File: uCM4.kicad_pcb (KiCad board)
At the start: 2 copper layers, 55 x 48 mm, 81 parts, among them IC1 MAX17048G+, J10 USB_C_Receptacle, J2 Micro_SD_Card_Det, J4 Conn_01x04, J5 DummyJ, J6 DummyJ, Q2 SI2369DS, SW1 SW_DIP_x01, SW3 SW_Push, SW4 SW_SPDT, U1 BNO055, U18 RT9742GGJ5, U2 SN74LVC1G07DBVR, U3 TPS3839DBZ, U4 TPS61022, U5 TPD2EUSB30, U6 TP4057, U7 HC-PM254-5.0H-2X7PS, U8 ADAU7002ACBZ-R7, U9 HC-PM254-5.0H-2X7PS

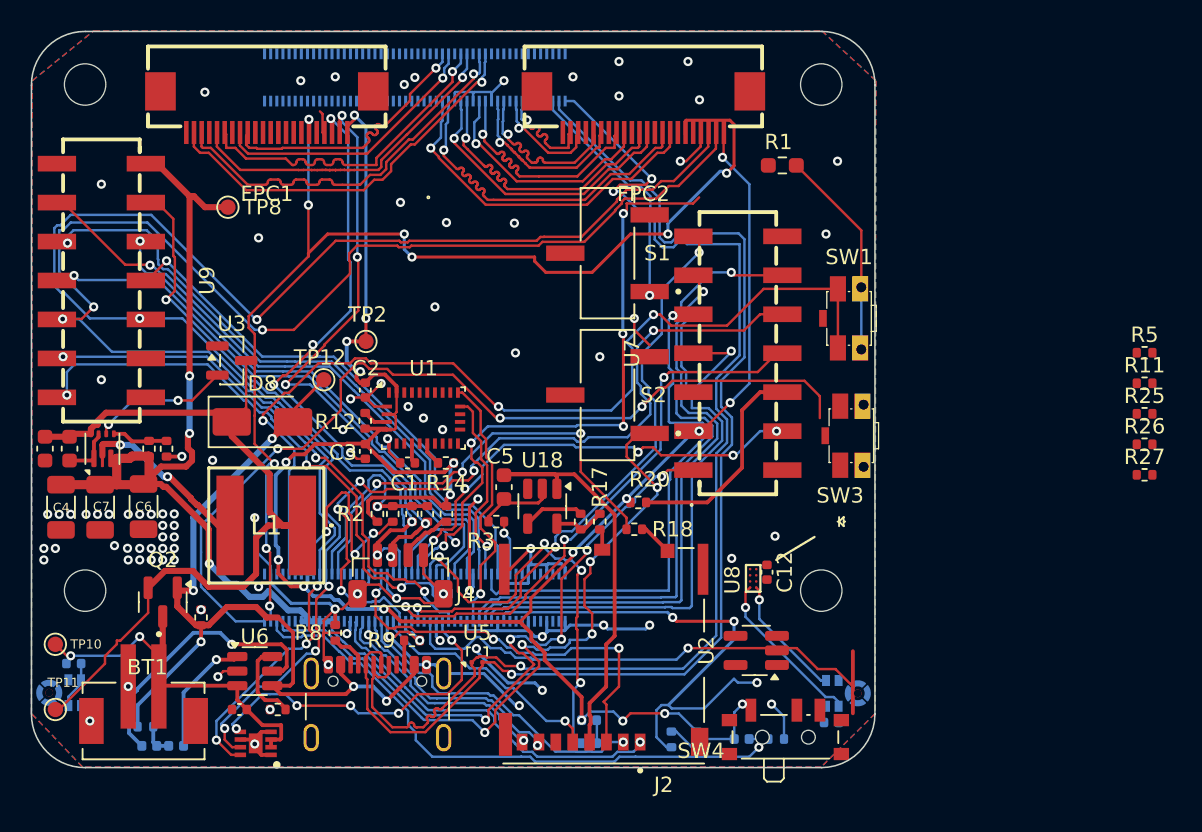
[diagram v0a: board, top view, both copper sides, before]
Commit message: Routing in progress
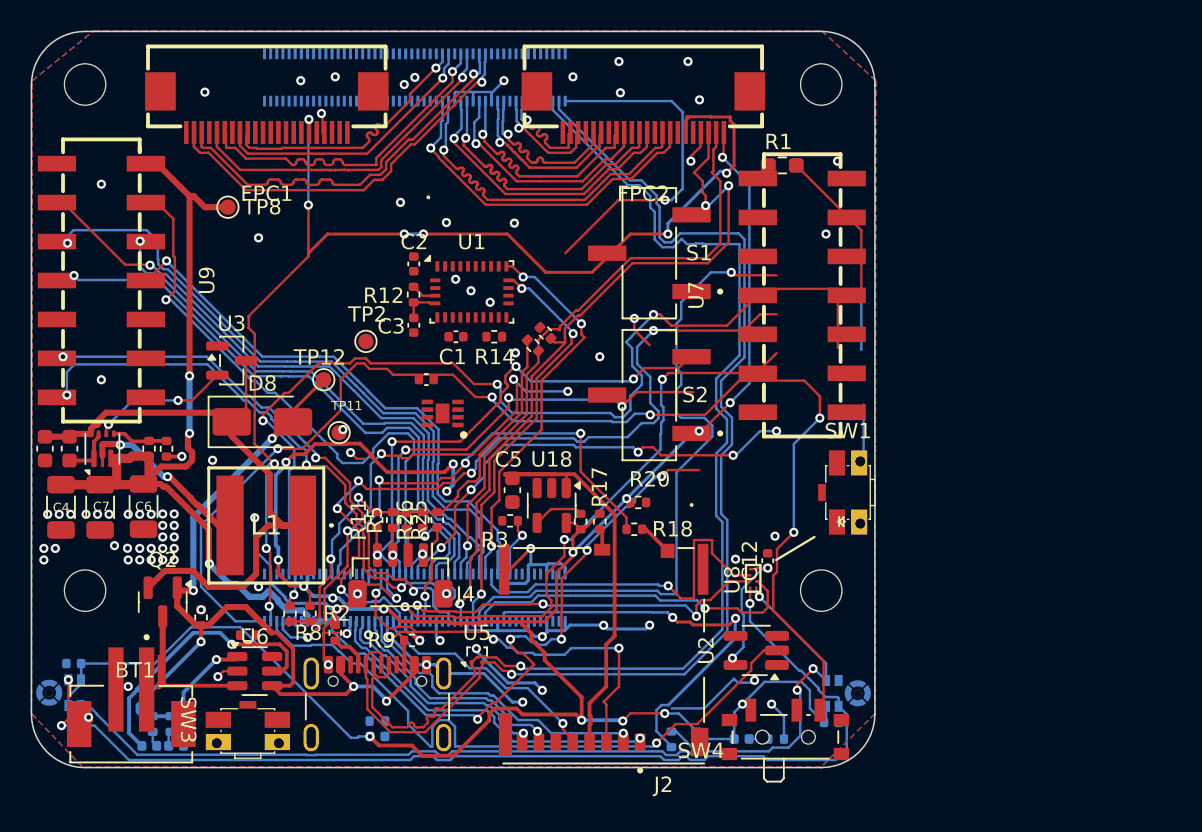
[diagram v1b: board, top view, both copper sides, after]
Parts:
- removed TP10: TestPoint, TestPoint:TestPoint_Pad_D1.0mm
- R27: moved to B.Cu
- moved R27 66.7 mm to (128.8, 130.2), turned to -90 degrees
- moved R11 50.9 mm to (143.4, 116.9), turned to 90 degrees
- moved R5 50.2 mm to (144.5, 116.9), turned to 90 degrees
- moved R26 47.3 mm to (146.4, 116.9), turned to 90 degrees
- moved R25 46.6 mm to (147.4, 116.9), turned to 90 degrees
- moved SW3 43.8 mm to (135.1, 130.7), turned to 0 degrees
- moved TP11 25.8 mm to (141.0, 111.2)
- moved C13 24.7 mm to (146.7, 107.7)
- moved IC1 24.7 mm to (147.8, 110.0)
- moved R7 14.7 mm to (154.4, 104.7), turned to 135 degrees
- moved R10 13.9 mm to (143.5, 130.0)
- moved D3 13.8 mm to (143.5, 131.0)
- moved R6 13.0 mm to (153.6, 105.5), turned to 135 degrees
- moved SW1 11.4 mm to (174.2, 115.1)
- moved R4 9.33 mm to (137.8, 123.0), turned to -90 degrees
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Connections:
- FPC2 pad 3: GND -> /SCL1
- Module1 pad 35: GND -> /SCL1
- R23 pad 1: +3V3 -> /GPIO_VREF
- R25 pad 2: Net-(R25-Pad2) -> /GPIO_VREF
- R26 pad 2: Net-(R25-Pad2) -> /GPIO_VREF
- R7 pad 1: GND -> /SCL1
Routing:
- net /SDA0: track 107.0 -> 0.00 mm, vias 6 -> 0
- net /SCL0: track 102.7 -> 0.00 mm, vias 5 -> 0
- net (no net): track 70.2 -> 0.00 mm, vias 4 -> 0
- net /PDM_CLK: track 10.7 -> 70.1 mm, vias 1 -> 3
- net /PDM_DAT: track 8.14 -> 63.4 mm, vias 1 -> 3
- net /SCL1: track 0.00 -> 47.2 mm, vias 0 -> 3
- net unconnected-(Module1A-GPIO27-Pad48): track 41.0 -> 0.00 mm, vias 5 -> 0
- net unconnected-(Module1A-GPIO21-Pad25): track 36.0 -> 0.00 mm, vias 1 -> 0
- net /BTN0: track 35.5 -> 0.00 mm, vias 1 -> 0
- net /SDA3: track 0.00 -> 35.1 mm, vias 0 -> 4
- net GND: track 131.7 -> 99.8 mm, vias 99 -> 85
- net /SCL3: track 0.00 -> 31.6 mm, vias 0 -> 4
- net +3V3: track 148.2 -> 170.5 mm
- net /BAT_ALERT: track 22.3 -> 0.00 mm, vias 5 -> 0
- net Net-(Module1A-Global_EN): track 59.3 -> 81.5 mm, vias 3 -> 5
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
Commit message: Routed and should be ready to order
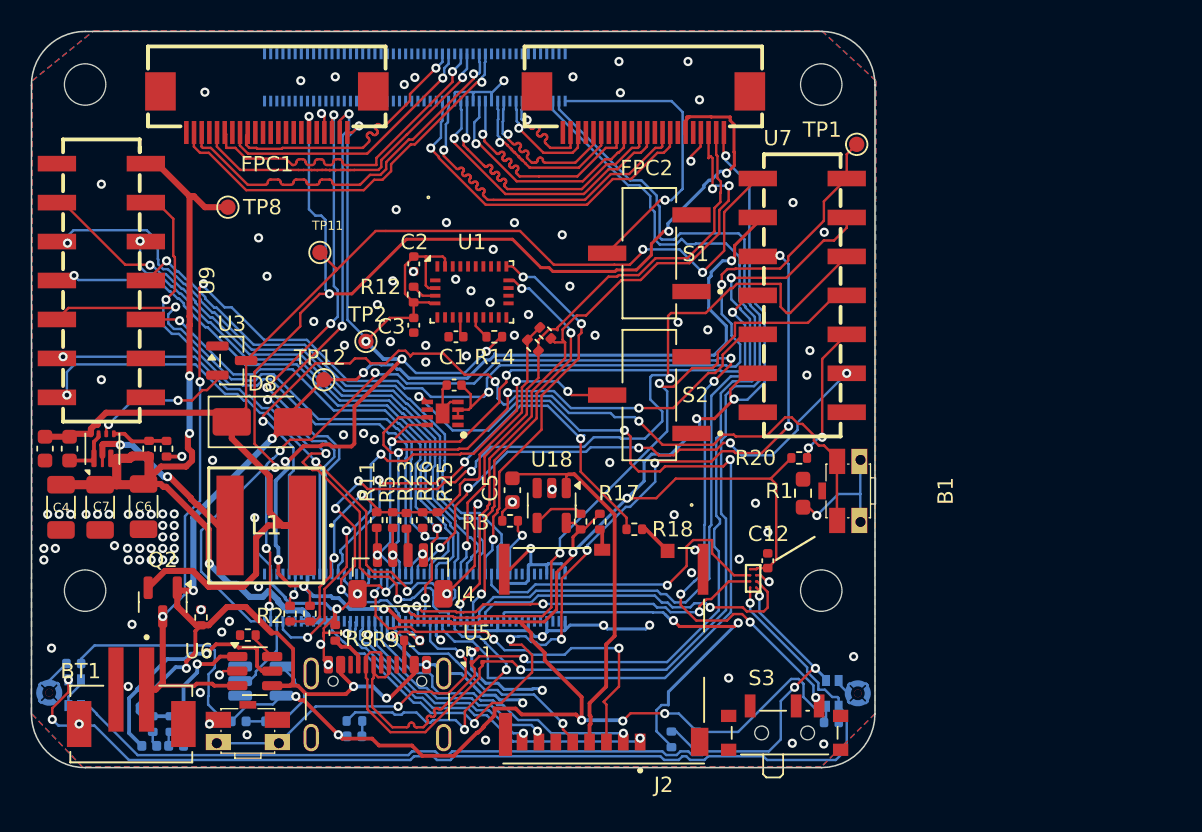
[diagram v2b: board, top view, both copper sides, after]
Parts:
- removed SW3: SW_Push, KiCAD_Randoms:PTS840_PM_SMTR_LFS
- removed SW4: SW_SPDT, Button_Switch_SMD:SW_SPDT_PCM12
- added B1: SW_DIP_x01, KiCAD_Randoms:PTS840_PM_SMTR_LFS, F.Cu at (174.2, 115.0)
- added B2: SW_Push, KiCAD_Randoms:PTS840_PM_SMTR_LFS, F.Cu at (135.1, 130.7)
- added TP1: TestPoint, TestPoint:TestPoint_Pad_D1.0mm, F.Cu at (174.8, 92.4)
- S3: renamed from SW1; value SW_DIP_x01 -> SW_SPDT; footprint KiCAD_Randoms:PTS840_PM_SMTR_LFS -> Button_Switch_SMD:SW_SPDT_PCM12
- U2: moved to B.Cu
- moved D1 32.8 mm to (134.4, 130.0)
- moved R13 32.8 mm to (136.7, 130.0)
- moved U2 32.4 mm to (135.9, 127.4), turned to 0 degrees
- moved R1 21.4 mm to (171.2, 115.2), turned to 90 degrees
- moved S3 15.9 mm to (170.1, 130.4), turned to 0 degrees
- moved TP11 11.8 mm to (139.8, 99.5)
- moved R20 10.9 mm to (171.0, 112.8)
- moved C13 1.85 mm to (148.5, 108.1)
- moved D3 1.50 mm to (142.0, 131.0)
- moved R10 1.50 mm to (142.0, 130.0)
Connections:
- R1 pad 1: Net-(R1-Pad1) -> Net-(B1-Pad1)
- S3 pad 1: Net-(R1-Pad1) -> unconnected-(S3-A-Pad1)
- S3 pad 2: /RESET -> GND
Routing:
- net /BAT: track 11.8 -> 98.7 mm, vias 0 -> 5
- net /BAT_ALERT: track 0.00 -> 59.2 mm, vias 0 -> 3
- net +3V3: track 170.5 -> 225.8 mm, vias 19 -> 18
- net /BOOST_IN: track 41.2 -> 85.7 mm, vias 1 -> 2
- net VBUS: track 56.0 -> 94.8 mm, vias 5 -> 7
- net /nPWR_LED: track 42.7 -> 5.24 mm, vias 1 -> 0
- net /SDA0: track 0.00 -> 36.6 mm, vias 0 -> 3
- net /SCL0: track 0.00 -> 35.9 mm, vias 0 -> 3
- net /SDA6: track 5.68 -> 40.4 mm, vias 1 -> 2
- net /SCL6: track 6.48 -> 34.2 mm, vias 1 -> 3
- net GND: track 99.8 -> 125.0 mm, vias 85 -> 127
- net /BTN0: track 0.00 -> 23.3 mm, vias 0 -> 2
- net +5V: track 97.8 -> 119.0 mm, vias 8 -> 10
- net /GPIO7: track 0.00 -> 18.9 mm, vias 0 -> 2
- net Net-(R1-Pad1): track 17.8 -> 0.00 mm
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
